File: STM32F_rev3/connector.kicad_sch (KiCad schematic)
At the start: 26 parts, among them J3 502225-0801, Q5 2N3904, Q6 IRF540N, Q7 IRF540N, U4 MIC2940A-3.3WU, U5 MIC2940A-5.0WT, U6 LT4363IMS, U7 MIC2940A-5.0WT

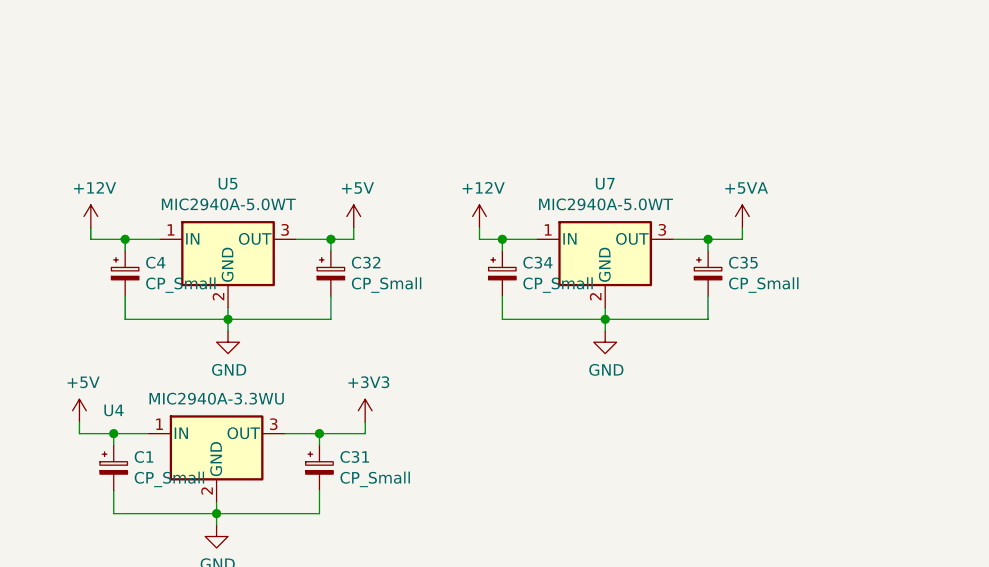
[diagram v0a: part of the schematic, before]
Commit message: Update on PMIC
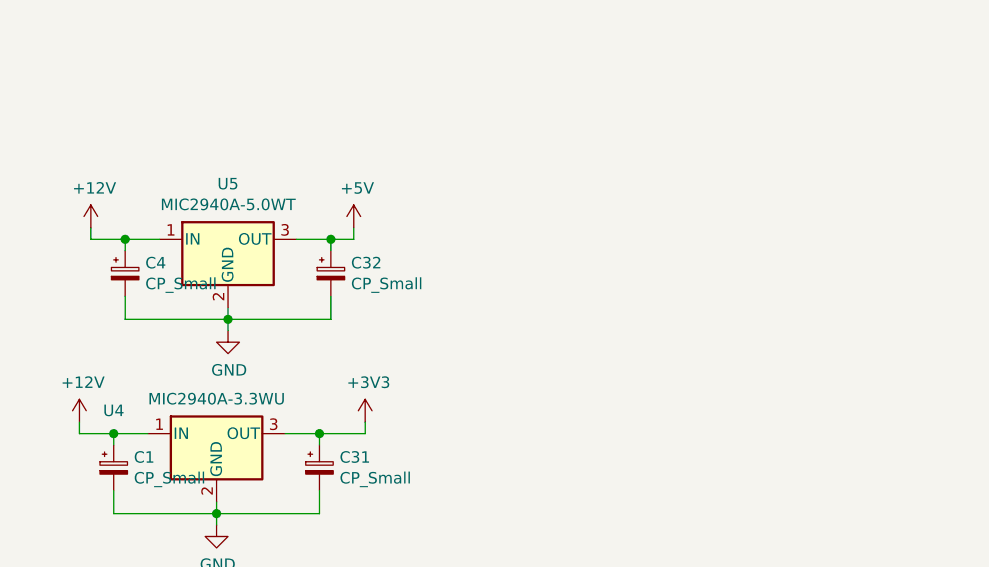
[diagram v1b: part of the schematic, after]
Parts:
- removed C34, C35: CP_Small, symbol Device:CP_Small
- removed U7: MIC2940A-5.0WT, Package_TO_SOT_THT:TO-220-3_Vertical, symbol Regulator_Linear:L7805
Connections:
- net +12V: now also C1.1, U4.1 (IN)
- net +5V: no longer C1.1, U4.1 (IN)
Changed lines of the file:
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@@
 (kicad_sch (version 20201015) (generator eeschema)
-  (page 1 5)
+  (page 1 6)
   (paper "A4")
   (junction (at 46.99 93.98) (diameter 1.016) (color 0 0 0 0))
@@
   (junction (at 82.55 109.22) (diameter 1.016) (color 0 0 0 0))
   (junction (at 91.44 93.98) (diameter 1.016) (color 0 0 0 0))
-  (junction (at 93.98 44.45) (diameter 1.016) (color 0 0 0 0))
   (junction (at 101.6 93.98) (diameter 1.016) (color 0 0 0 0))
-  (junction (at 105.41 53.34) (diameter 1.016) (color 0 0 0 0))
   (junction (at 105.41 93.98) (diameter 1.016) (color 0 0 0 0))
   (junction (at 105.41 104.14) (diameter 1.016) (color 0 0 0 0))
-  (junction (at 116.84 44.45) (diameter 1.016) (color 0 0 0 0))
   (junction (at 119.38 121.92) (diameter 1.016) (color 0 0 0 0))
   (junction (at 185.42 66.04) (diameter 1.016) (color 0 0 0 0))
@@
   (junction (at 247.65 111.76) (diameter 1.016) (color 0 0 0 0))
   (junction (at 247.65 114.3) (diameter 1.016) (color 0 0 0 0))
-  (no_connect (at 113.03 127))
+  (no_connect (at 113.03 119.38))
   (no_connect (at 231.14 91.44))
   (no_connect (at 231.14 106.68))
-  (no_connect (at 231.14 83.82))
-  (no_connect (at 113.03 116.84))
-  (no_connect (at 90.17 127))
-  (no_connect (at 231.14 78.74))
+  (no_connect (at 231.14 86.36))
   (no_connect (at 231.14 99.06))
-  (no_connect (at 231.14 76.2))
+  (no_connect (at 113.03 124.46))
+  (no_connect (at 231.14 88.9))
   (no_connect (at 231.14 109.22))
   (no_connect (at 231.14 96.52))
-  (no_connect (at 231.14 88.9))
+  (no_connect (at 231.14 114.3))
+  (no_connect (at 231.14 93.98))
   (no_connect (at 231.14 111.76))
-  (no_connect (at 231.14 86.36))
-  (no_connect (at 113.03 119.38))
-  (no_connect (at 231.14 93.98))
-  (no_connect (at 231.14 114.3))
+  (no_connect (at 231.14 104.14))
+  (no_connect (at 231.14 78.74))
+  (no_connect (at 90.17 127))
+  (no_connect (at 113.03 127))
+  (no_connect (at 113.03 116.84))
+  (no_connect (at 231.14 76.2))
+  (no_connect (at 231.14 101.6))
+  (no_connect (at 231.14 83.82))
   (no_connect (at 231.14 81.28))
-  (no_connect (at 113.03 124.46))
-  (no_connect (at 231.14 104.14))
-  (no_connect (at 231.14 101.6))
   (wire (pts (xy 46.99 64.77) (xy 46.99 66.04))
     (stroke (width 0) (type solid) (color 0 0 0 0))
@@
     (stroke (width 0) (type solid) (color 0 0 0 0))
   )
-  (wire (pts (xy 91.44 43.18) (xy 91.44 44.45))
-    (stroke (width 0) (type solid) (color 0 0 0 0))
-  )
-  (wire (pts (xy 91.44 44.45) (xy 93.98 44.45))
-    (stroke (width 0) (type solid) (color 0 0 0 0))
-  )
   (wire (pts (xy 91.44 93.98) (xy 93.98 93.98))
     (stroke (width 0) (type solid) (color 0 0 0 0))
@@
     (stroke (width 0) (type solid) (color 0 0 0 0))
   )
-  (wire (pts (xy 93.98 44.45) (xy 93.98 45.72))
-    (stroke (width 0) (type solid) (color 0 0 0 0))
-  )
-  (wire (pts (xy 93.98 50.8) (xy 93.98 53.34))
-    (stroke (width 0) (type solid) (color 0 0 0 0))
-  )
-  (wire (pts (xy 93.98 53.34) (xy 105.41 53.34))
-    (stroke (width 0) (type solid) (color 0 0 0 0))
-  )
-  (wire (pts (xy 97.79 44.45) (xy 93.98 44.45))
-    (stroke (width 0) (type solid) (color 0 0 0 0))
-  )
   (wire (pts (xy 99.06 93.98) (xy 101.6 93.98))
     (stroke (width 0) (type solid) (color 0 0 0 0))
@@
     (stroke (width 0) (type solid) (color 0 0 0 0))
   )
-  (wire (pts (xy 105.41 52.07) (xy 105.41 53.34))
-    (stroke (width 0) (type solid) (color 0 0 0 0))
-  )
-  (wire (pts (xy 105.41 53.34) (xy 105.41 54.61))
-    (stroke (width 0) (type solid) (color 0 0 0 0))
-  )
   (wire (pts (xy 105.41 93.98) (xy 105.41 95.25))
     (stroke (width 0) (type solid) (color 0 0 0 0))
@@
     (stroke (width 0) (type solid) (color 0 0 0 0))
   )
-  (wire (pts (xy 113.03 44.45) (xy 116.84 44.45))
-    (stroke (width 0) (type solid) (color 0 0 0 0))
-  )
   (wire (pts (xy 113.03 114.3) (xy 125.73 114.3))
     (stroke (width 0) (type solid) (color 0 0 0 0))
@@
     (stroke (width 0) (type solid) (color 0 0 0 0))
   )
-  (wire (pts (xy 116.84 44.45) (xy 116.84 45.72))
-    (stroke (width 0) (type solid) (color 0 0 0 0))
-  )
-  (wire (pts (xy 116.84 50.8) (xy 116.84 53.34))
-    (stroke (width 0) (type solid) (color 0 0 0 0))
-  )
-  (wire (pts (xy 116.84 53.34) (xy 105.41 53.34))
-    (stroke (width 0) (type solid) (color 0 0 0 0))
-  )
   (wire (pts (xy 119.38 91.44) (xy 119.38 93.98))
     (stroke (width 0) (type solid) (color 0 0 0 0))
@@
     (stroke (width 0) (type solid) (color 0 0 0 0))
   )
-  (wire (pts (xy 120.65 43.18) (xy 120.65 44.45))
-    (stroke (width 0) (type solid) (color 0 0 0 0))
-  )
-  (wire (pts (xy 120.65 44.45) (xy 116.84 44.45))
-    (stroke (width 0) (type solid) (color 0 0 0 0))
-  )
   (wire (pts (xy 125.73 114.3) (xy 125.73 124.46))
     (stroke (width 0) (type solid) (color 0 0 0 0))
@@
     (effects (font (size 1.27 1.27)) (justify right))
   )
-  (symbol (lib_id "power:+5V") (at 46.99 64.77 0) (unit 1)
-    (in_bom yes) (on_board yes)
-    (property "Reference" "#PWR09" (id 0) (at 46.99 68.58 0)
-      (effects (font (size 1.27 1.27)) hide)
-    )
-    (property "Value" "+5V" (id 1) (at 47.371 60.3758 0))
+  (symbol (lib_id "power:+12V") (at 46.99 64.77 0) (unit 1)
+    (in_bom yes) (on_board yes)
+    (property "Reference" "#PWR0137" (id 0) (at 46.99 68.58 0)
+      (effects (font (size 1.27 1.27)) hide)
+    )
+    (property "Value" "+12V" (id 1) (at 47.371 60.3758 0))
     (property "Footprint" "" (id 2) (at 46.99 64.77 0)
       (effects (font (size 1.27 1.27)) hide)
@@
     )
   )
-  (symbol (lib_id "power:+12V") (at 91.44 43.18 0) (unit 1)
-    (in_bom yes) (on_board yes)
-    (property "Reference" "#PWR019" (id 0) (at 91.44 46.99 0)
-      (effects (font (size 1.27 1.27)) hide)
-    )
-    (property "Value" "+12V" (id 1) (at 91.821 38.7858 0))
-    (property "Footprint" "" (id 2) (at 91.44 43.18 0)
-      (effects (font (size 1.27 1.27)) hide)
-    )
-    (property "Datasheet" "" (id 3) (at 91.44 43.18 0)
-      (effects (font (size 1.27 1.27)) hide)
-    )
-  )
   (symbol (lib_id "power:+12V") (at 119.38 91.44 0) (unit 1)
     (in_bom yes) (on_board yes)
@@
     )
   )
-  (symbol (lib_id "power:+5VA") (at 120.65 43.18 0) (unit 1)
-    (in_bom yes) (on_board yes)
-    (property "Reference" "#PWR0164" (id 0) (at 120.65 46.99 0)
-      (effects (font (size 1.27 1.27)) hide)
-    )
-    (property "Value" "+5VA" (id 1) (at 121.031 38.7858 0))
-    (property "Footprint" "" (id 2) (at 120.65 43.18 0)
-      (effects (font (size 1.27 1.27)) hide)
-    )
-    (property "Datasheet" "" (id 3) (at 120.65 43.18 0)
-      (effects (font (size 1.27 1.27)) hide)
-    )
-  )
   (symbol (lib_id "power:+12VA") (at 185.42 63.5 0) (unit 1)
     (in_bom yes) (on_board yes)
@@
     )
     (property "Datasheet" "" (id 3) (at 74.93 120.65 0)
-      (effects (font (size 1.27 1.27)) hide)
-    )
-  )
-  (symbol (lib_id "power:GND") (at 105.41 54.61 0) (unit 1)
-    (in_bom yes) (on_board yes)
-    (property "Reference" "#PWR020" (id 0) (at 105.41 60.96 0)
-      (effects (font (size 1.27 1.27)) hide)
-    )
-    (property "Value" "GND" (id 1) (at 105.537 59.0042 0))
-    (property "Footprint" "" (id 2) (at 105.41 54.61 0)
-      (effects (font (size 1.27 1.27)) hide)
-    )
-    (property "Datasheet" "" (id 3) (at 105.41 54.61 0)
       (effects (font (size 1.27 1.27)) hide)
     )
@@
     )
     (property "Datasheet" "~" (id 3) (at 74.93 48.26 0)
-      (effects (font (size 1.27 1.27)) hide)
-    )
-  )
-  (symbol (lib_id "Device:CP_Small") (at 93.98 48.26 0) (unit 1)
-    (in_bom yes) (on_board yes)
-    (property "Reference" "C34" (id 0) (at 96.2152 47.0916 0)
-      (effects (font (size 1.27 1.27)) (justify left))
-    )
-    (property "Value" "CP_Small" (id 1) (at 96.2152 49.403 0)
-      (effects (font (size 1.27 1.27)) (justify left))
-    )
-    (property "Footprint" "" (id 2) (at 93.98 48.26 0)
-      (effects (font (size 1.27 1.27)) hide)
-    )
-    (property "Datasheet" "~" (id 3) (at 93.98 48.26 0)
-      (effects (font (size 1.27 1.27)) hide)
-    )
-  )
-  (symbol (lib_id "Device:CP_Small") (at 116.84 48.26 0) (unit 1)
-    (in_bom yes) (on_board yes)
-    (property "Reference" "C35" (id 0) (at 119.0752 47.0916 0)
-      (effects (font (size 1.27 1.27)) (justify left))
-    )
-    (property "Value" "CP_Small" (id 1) (at 119.0752 49.403 0)
-      (effects (font (size 1.27 1.27)) (justify left))
-    )
-    (property "Footprint" "" (id 2) (at 116.84 48.26 0)
-      (effects (font (size 1.27 1.27)) hide)
-    )
-    (property "Datasheet" "~" (id 3) (at 116.84 48.26 0)
       (effects (font (size 1.27 1.27)) hide)
     )
@@
       (effects (font (size 1.27 1.27)) hide)
     )
-  )
-  (symbol (lib_id "Regulator_Linear:L7805") (at 105.41 44.45 0) (unit 1)
-    (in_bom yes) (on_board yes)
-    (property "Reference" "U7" (id 0) (at 105.41 38.3032 0))
-    (property "Value" "MIC2940A-5.0WT" (id 1) (at 105.41 40.6146 0))
-    (property "Footprint" "Package_TO_SOT_THT:TO-220-3_Vertical" (id 2) (at 106.045 48.26 0)
-      (effects (font (size 1.27 1.27) italic) (justify left) hide)
-    )
-    (property "Datasheet" "http://www.st.com/content/ccc/resource/technical/document/datasheet/41/4f/b3/b0/12/d4/47/88/CD00000444.pdf/files/CD00000444.pdf/jcr:content/translations/en.CD00000444.pdf" (id 3) (at 105.41 45.72 0)
-      (effects (font (size 1.27 1.27)) hide)
-    )
-    (property "DIGY" "576-1136-ND" (id 4) (at 105.41 44.45 0)
-      (effects (font (size 1.27 1.27)) hide)
-    )

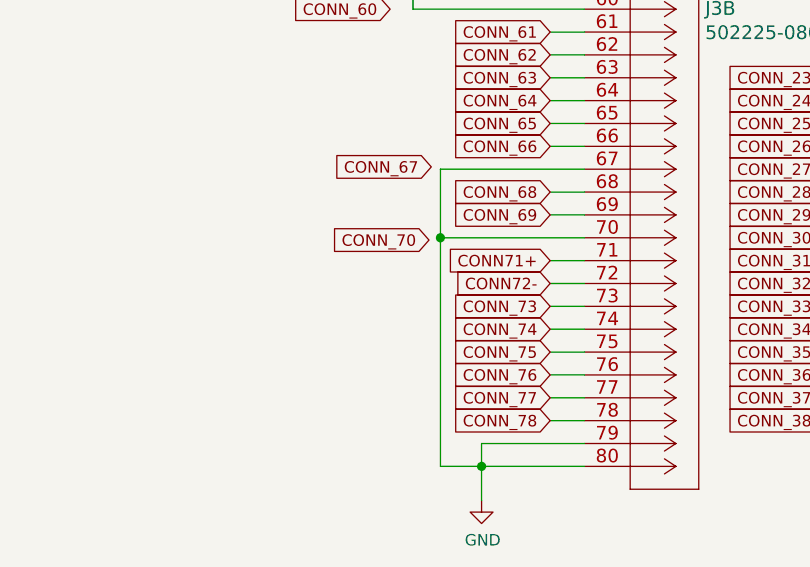
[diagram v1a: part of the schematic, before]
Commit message: GPIO
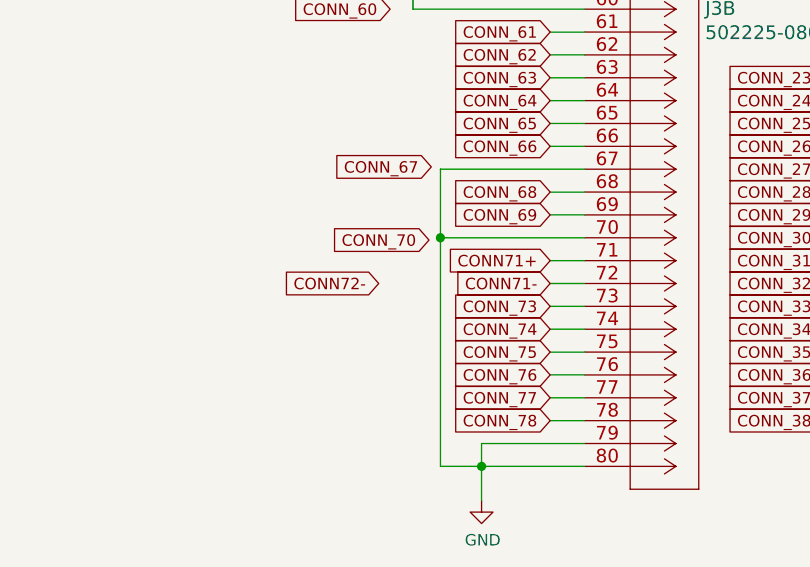
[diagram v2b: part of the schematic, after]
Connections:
- net CONN72-: no longer J3.72
- new net CONN71-: J3.72
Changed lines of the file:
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@@
   (junction (at 247.65 111.76) (diameter 1.016) (color 0 0 0 0))
   (junction (at 247.65 114.3) (diameter 1.016) (color 0 0 0 0))
-  (no_connect (at 113.03 119.38))
-  (no_connect (at 231.14 91.44))
-  (no_connect (at 231.14 106.68))
-  (no_connect (at 231.14 86.36))
-  (no_connect (at 231.14 99.06))
-  (no_connect (at 113.03 124.46))
+  (no_connect (at 231.14 83.82))
   (no_connect (at 231.14 88.9))
-  (no_connect (at 231.14 109.22))
-  (no_connect (at 231.14 96.52))
-  (no_connect (at 231.14 114.3))
-  (no_connect (at 231.14 93.98))
-  (no_connect (at 231.14 111.76))
   (no_connect (at 231.14 104.14))
   (no_connect (at 231.14 78.74))
+  (no_connect (at 231.14 81.28))
+  (no_connect (at 231.14 91.44))
+  (no_connect (at 231.14 109.22))
+  (no_connect (at 231.14 101.6))
   (no_connect (at 90.17 127))
+  (no_connect (at 231.14 93.98))
+  (no_connect (at 231.14 114.3))
+  (no_connect (at 231.14 106.68))
+  (no_connect (at 231.14 99.06))
+  (no_connect (at 231.14 96.52))
+  (no_connect (at 231.14 111.76))
+  (no_connect (at 113.03 124.46))
+  (no_connect (at 231.14 76.2))
+  (no_connect (at 113.03 116.84))
+  (no_connect (at 231.14 86.36))
   (no_connect (at 113.03 127))
-  (no_connect (at 113.03 116.84))
-  (no_connect (at 231.14 76.2))
-  (no_connect (at 231.14 101.6))
-  (no_connect (at 231.14 83.82))
-  (no_connect (at 231.14 81.28))
+  (no_connect (at 113.03 119.38))
   (wire (pts (xy 46.99 64.77) (xy 46.99 66.04))
     (stroke (width 0) (type solid) (color 0 0 0 0))
@@
     (stroke (width 0) (type solid) (color 0 0 0 0))
   )
+  (global_label "CONN72-" (shape input) (at 181.61 99.06 180)
+    (effects (font (size 1.27 1.27)) (justify right))
+  )
   (global_label "CONN_59" (shape input) (at 182.88 66.04 180)
     (effects (font (size 1.27 1.27)) (justify right))
@@
     (effects (font (size 1.27 1.27)) (justify right))
   )
-  (global_label "CONN72-" (shape input) (at 200.66 99.06 180)
-    (effects (font (size 1.27 1.27)) (justify right))
-  )
+  (global_label "CONN71-" (shape input) (at 200.66 99.06 180)
+    (effects (font (size 1.27 1.27)) (justify right))
+  )
